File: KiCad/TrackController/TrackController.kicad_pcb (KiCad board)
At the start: 2 copper layers, 133.5 x 74 mm, 3 parts, among them J1 DE9_Plug_MountingHoles, U1 mini ESP32, U2 TXS0108EPW

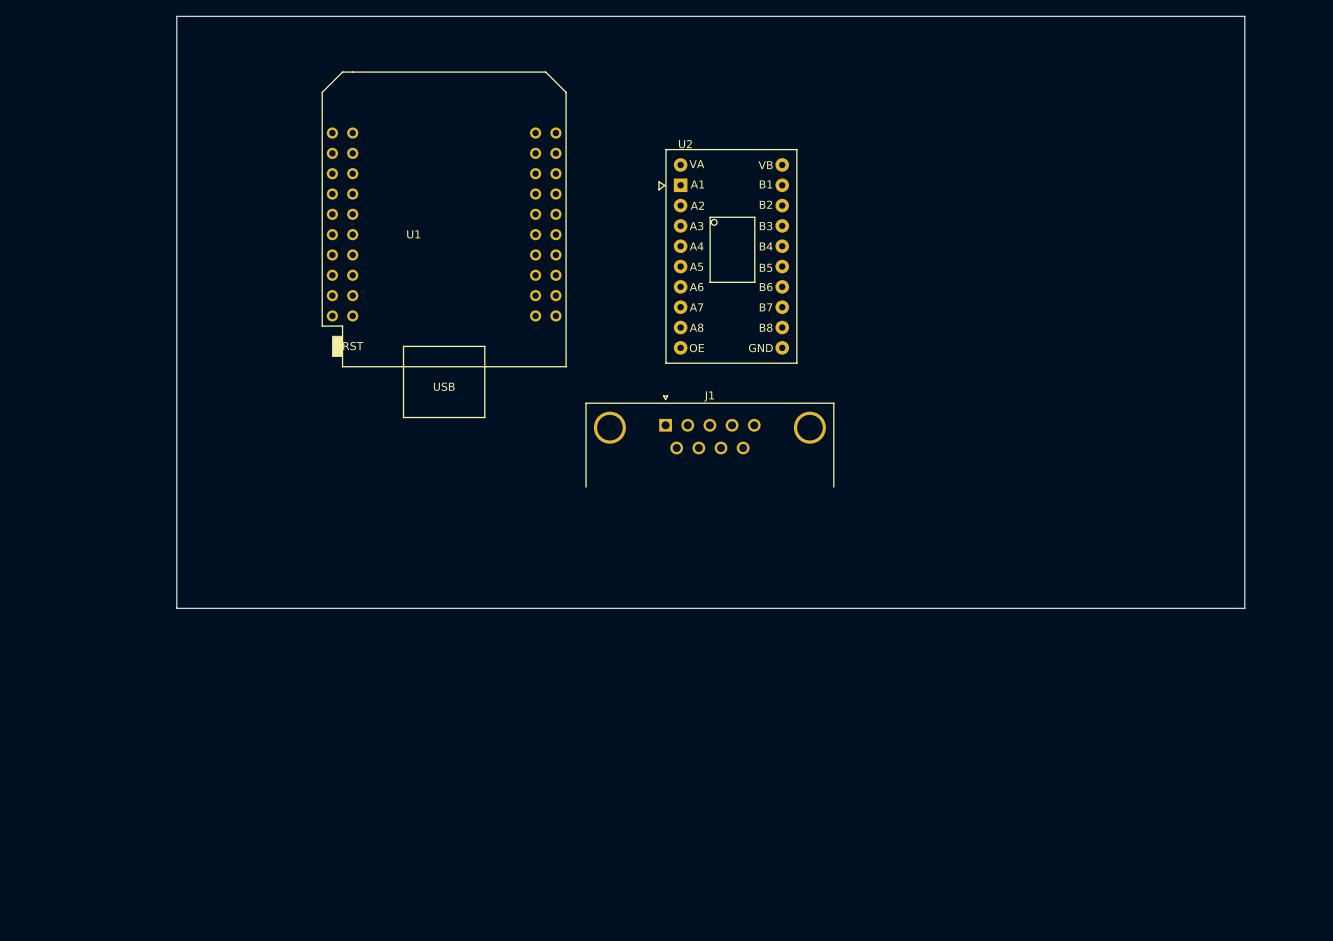
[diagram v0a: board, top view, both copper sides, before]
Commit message: Added KiCAD pcb design
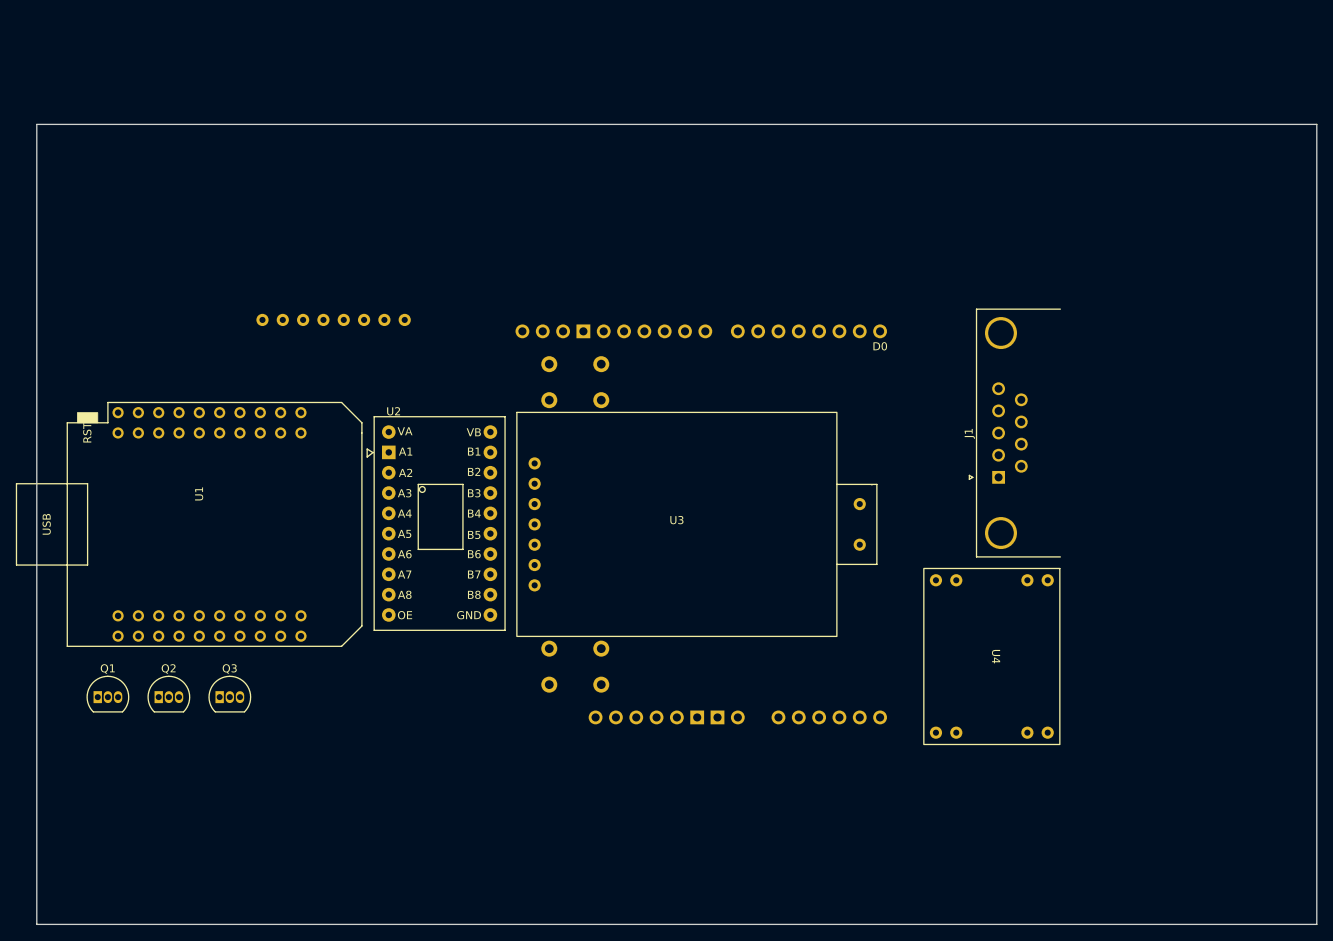
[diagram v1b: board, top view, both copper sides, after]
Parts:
- added A1: Arduino_Uno_R3_Shield, PCM_arduino-library:Arduino_Uno_R3_Shield, F.Cu at (81.9, 126.7)
- added LCD1: ~, railtrack:1.77 LCD Display 128x160, B.Cu at (77.1, 94.0)
- added Q1: BC547, Package_TO_SOT_THT:TO-92_Inline, F.Cu at (47.6, 121.6)
- added Q2: BC547, Package_TO_SOT_THT:TO-92_Inline, F.Cu at (55.2, 121.6)
- added Q3: BC547, Package_TO_SOT_THT:TO-92_Inline, F.Cu at (62.9, 121.6)
- added SW1: SW_Push, Button_Switch_THT:SW_PUSH_6mm, B.Cu at (104.1, 120.0)
- added SW2: SW_Push, Button_Switch_THT:SW_PUSH_6mm, B.Cu at (110.6, 80.0)
- added U3: ~, railtrack:MCP2515 Module, F.Cu at (120.0, 100.0)
- added U4: ~, railtrack:MP1484 Module, F.Cu at (159.4, 116.5)
- U1: value mini ESP32 -> mini_esp32
- moved U2 49.5 mm to (84.0, 91.0)
- moved U1 47.6 mm to (61.6, 100.0), turned to -90 degrees
- moved J1 42.1 mm to (160.2, 94.1), turned to 90 degrees
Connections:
- U1 pad 1: (no net) -> GND
- U1 pad 10: (no net) -> unconnected-(U1-IO_19/D6-Pad10)
- U1 pad 11: (no net) -> unconnected-(U1-IO_34-Pad11)
- U1 pad 12: (no net) -> unconnected-(U1-IO_23/D7-Pad12)
- U1 pad 13: (no net) -> unconnected-(U1-IO_14/TMS-Pad13)
- U1 pad 14: (no net) -> unconnected-(U1-IO_05/D8-Pad14)
- U1 pad 15: (no net) -> unconnected-(U1-NC-Pad15)
- U1 pad 16: (no net) -> /3V3
- U1 pad 17: (no net) -> unconnected-(U1-IO_09/SD2-Pad17)
- U1 pad 18: (no net) -> unconnected-(U1-IO_13/TCK-Pad18)
- U1 pad 19: (no net) -> unconnected-(U1-CMD-Pad19)
- U1 pad 2: (no net) -> unconnected-(U1-RST-Pad2)
- U1 pad 20: (no net) -> unconnected-(U1-IO_10/SD3-Pad20)
- U1 pad 21: (no net) -> unconnected-(U1-TXD-Pad21)
- U1 pad 22: (no net) -> GND
- U1 pad 23: (no net) -> unconnected-(U1-RXD-Pad23)
- U1 pad 24: (no net) -> unconnected-(U1-IO_27-Pad24)
- U1 pad 25: (no net) -> unconnected-(U1-IO_22/D1/SCL-Pad25)
- U1 pad 26: (no net) -> unconnected-(U1-IO_25-Pad26)
- U1 pad 27: (no net) -> unconnected-(U1-IO_21/D2/SDA-Pad27)
- U1 pad 28: (no net) -> unconnected-(U1-IO_32-Pad28)
- U1 pad 29: (no net) -> unconnected-(U1-IO_17/D3-Pad29)
- U1 pad 3: (no net) -> unconnected-(U1-NC-Pad3)
- U1 pad 30: (no net) -> unconnected-(U1-IO_12/TDI-Pad30)
- U1 pad 31: (no net) -> unconnected-(U1-IO_16/D4-Pad31)
- U1 pad 32: (no net) -> unconnected-(U1-IO_04-Pad32)
- U1 pad 33: (no net) -> GND
- U1 pad 34: (no net) -> unconnected-(U1-IO_00-Pad34)
- U1 pad 35: (no net) -> /VCC
- U1 pad 36: (no net) -> unconnected-(U1-IO_02-Pad36)
- U1 pad 37: (no net) -> unconnected-(U1-TD0-Pad37)
- U1 pad 38: (no net) -> unconnected-(U1-SD1-Pad38)
- U1 pad 39: (no net) -> unconnected-(U1-SD0-Pad39)
- U1 pad 4: (no net) -> unconnected-(U1-IO_36/SVP/A0-Pad4)
- U1 pad 40: (no net) -> unconnected-(U1-CLK-Pad40)
- U1 pad 5: (no net) -> unconnected-(U1-IO_39/SVN-Pad5)
- U1 pad 6: (no net) -> unconnected-(U1-IO_26/D0-Pad6)
- U1 pad 7: (no net) -> unconnected-(U1-IO_35-Pad7)
- U1 pad 8: (no net) -> unconnected-(U1-IO_18/D5-Pad8)
- U1 pad 9: (no net) -> unconnected-(U1-IO_33-Pad9)
- U2 pad 11: unconnected-(U2-GND-Pad11) -> GND
- U2 pad 19: unconnected-(U2-VCCB-Pad19) -> /VCC
- U2 pad 2: unconnected-(U2-VCCA-Pad2) -> /3V3
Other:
- board size 133.5 x 74 mm -> 160 x 100 mm
